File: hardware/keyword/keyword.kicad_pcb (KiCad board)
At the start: 4 copper layers, 44.4 x 19.3 mm, 81 parts, among them CN1 YZ00615050R-08, CN2 YZ00615050R-08, CN3 YZ00615050R-08, CN4 YZ00615050R-08, CN5 YZ00615050R-08, CN6 YZ00615050R-08, CN7 YZ00615050R-08, CN8 YZ00615050R-08, CN9 YZ00615050R-08, U10 W25Q16JVUXIQ, U11 STM32WB55RGVx, U12 MLPF-WB-04D3, U13 YZ13515055F-02025-02, U14 XL-1608RGBC, U15 YZ13515055F-02025-02, U16 XRTC252012S2R2MBCA, U17 SZYY0402Y_C434450, U18 TPS631000DRLR, U19 YZ37215050R-02025-05, U2 TPD2EUSB30, U20 YZ37215050R-02025-05, U3 NX2012SA-32.768KHZ-STD-MUB-2, U4 YZ13515055F-02025-02, U5 YZ13515055F-02025-02, U6 YZ13515055F-02025-02, U7 YZ13515055F-02025-02, U8 BQ25895RTW, U9 DFE252012P-1R0M=P2, X1 NX2016SA-32MHZ-STD-CZS-5

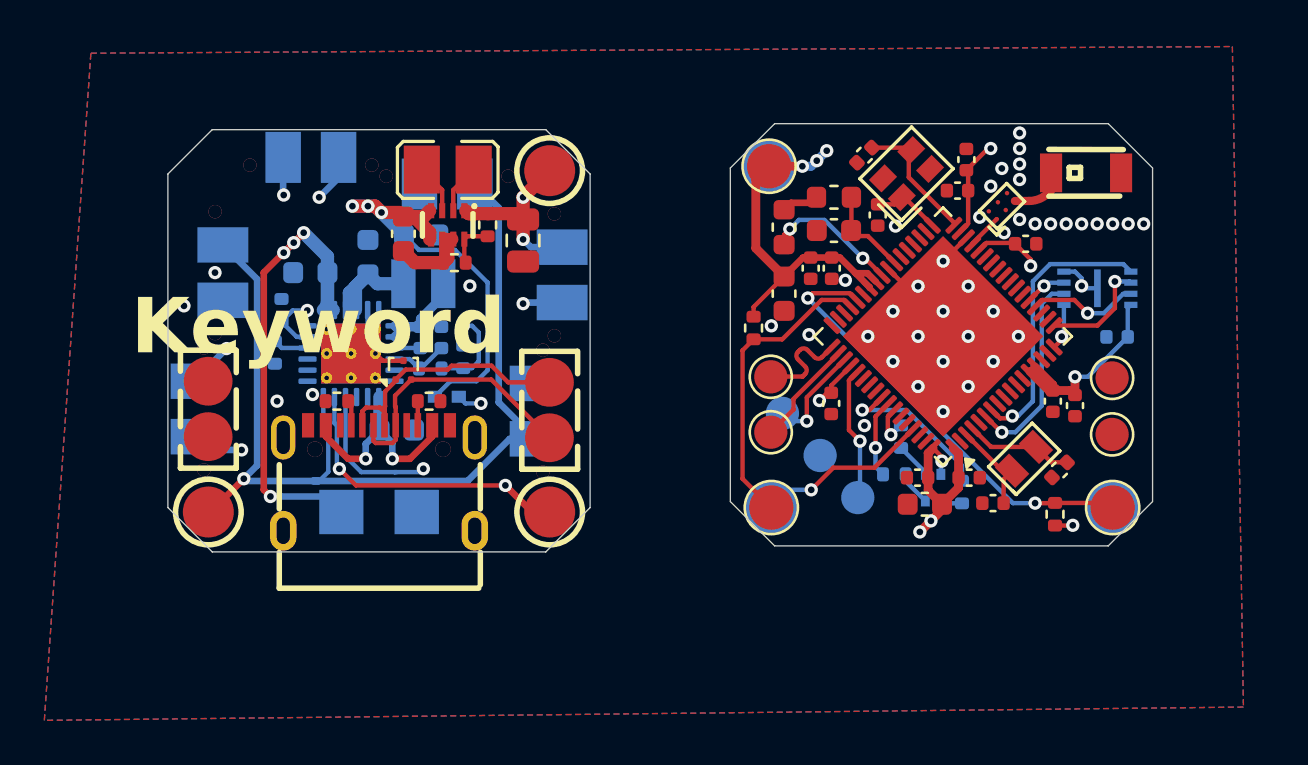
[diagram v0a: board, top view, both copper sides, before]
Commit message: finish case and stuff
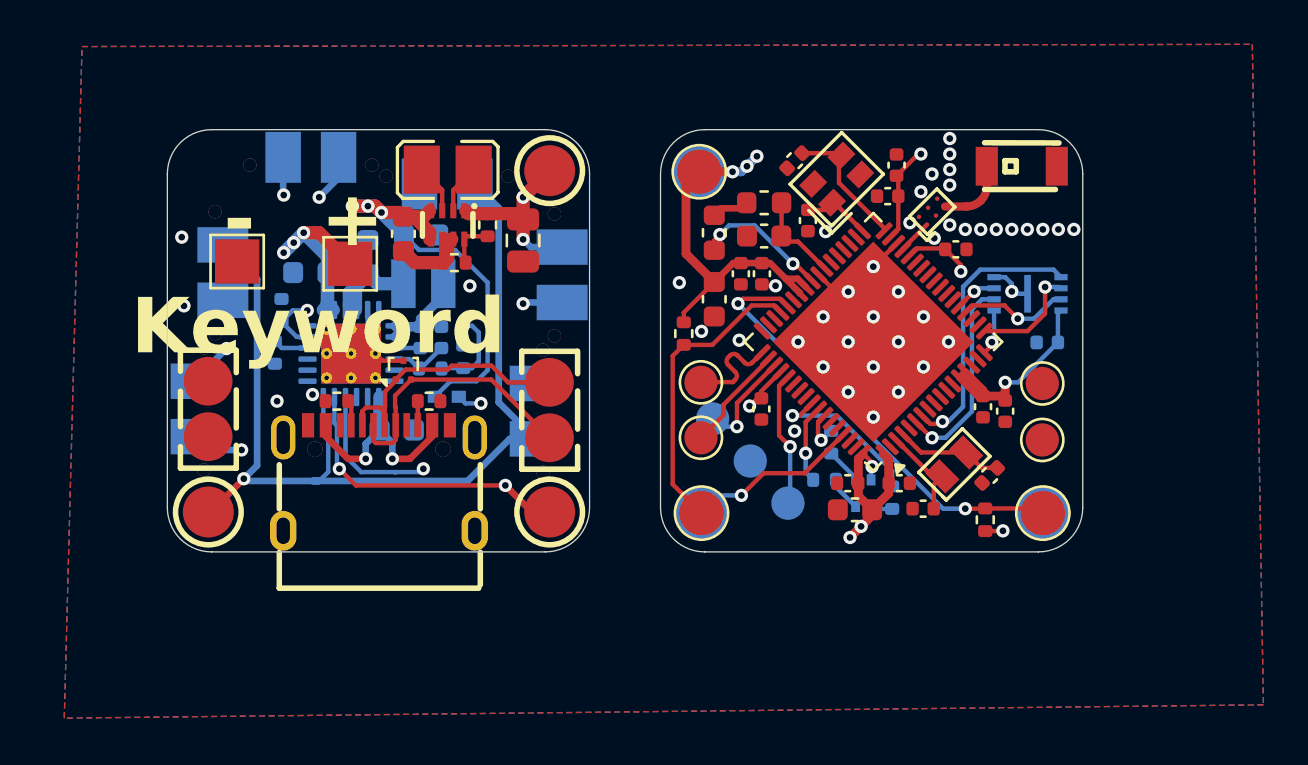
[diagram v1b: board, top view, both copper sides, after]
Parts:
- TP4, TP5: moved to F.Cu
- moved TP5 13.9 mm to (181.1, 78.5), turned to 90 degrees
- moved TP4 11.2 mm to (186.2, 78.6), turned to -90 degrees
- moved C1 3.16 mm to (206.8, 76.7)
- moved C2 3.16 mm to (206.2, 74.0)
- moved C24 3.16 mm to (204.9, 77.3)
- moved C25 3.16 mm to (213.5, 78.0)
- moved C26 3.16 mm to (204.8, 79.0)
- moved C27 3.16 mm to (211.0, 88.5)
- moved C28 3.16 mm to (202.6, 80.2)
- moved C29 3.16 mm to (203.8, 79.0)
- moved C3 3.16 mm to (217.7, 82.2)
- moved C31 3.16 mm to (209.0, 89.7)
- moved C32 3.16 mm to (210.8, 74.2)
- moved C33 3.16 mm to (210.4, 75.5)
- moved C34 3.16 mm to (214.8, 85.0)
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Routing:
- net Net-(C18-Pad1): track 23.3 -> 9.76 mm, vias 4 -> 3
- net Net-(AE1-ANT): track 2.56 -> 3.30 mm
- net GND: vias 44 -> 45
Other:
- board size 44.4 x 19.3 mm -> 41.3 x 19 mm
- board text added: "+"
- board text added: "-"
